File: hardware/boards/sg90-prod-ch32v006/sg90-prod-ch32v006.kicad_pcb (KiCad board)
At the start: 4 copper layers, 12.1 x 9.6 mm, 32 parts, among them J1 Servo Input, J2 Motor, J3 Debug, J4 Potentiometer, U1 H7133-1, U4 DRV8837, U5 CH32V006F8U6, U6 74LVC2G241GS,115

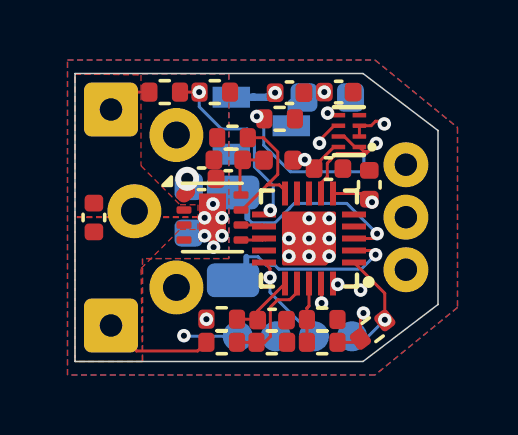
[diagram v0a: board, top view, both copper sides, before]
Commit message: rebuilt board
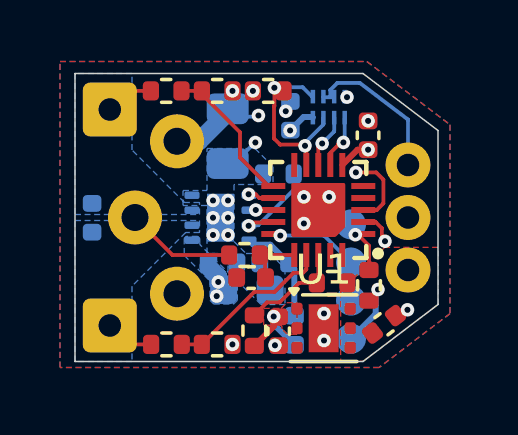
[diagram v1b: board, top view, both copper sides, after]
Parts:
- removed C3: 10µF, Capacitor_SMD:C_0402_1005Metric
- C1: value 10µF -> 1µF; footprint Capacitor_SMD:C_0603_1608Metric -> Capacitor_SMD:C_0402_1005Metric; moved to F.Cu
- C2: value 1µF -> 4.7µF
- C4, C7, C8, C9, FB1, R3, U4, U6: moved to B.Cu
- J4: moved to F.Cu
- NT1, NT2: footprint shared:NetTie-2_SMD_0.2mm -> shared:NetTie-2_SMD_0.127mm
- RS1: value 0.1Ω 1% -> 10mΩ 1%; footprint Resistor_SMD:R_1206_3216Metric -> Resistor_SMD:R_0805_2012Metric
- U1: value H7133-1 -> TLV76733DRVR; footprint shared:SOT-23-3_L2.9-W1.3-P1.90-LS2.4-BR -> Package_SON:WSON-6-1EP_2x2mm_P0.65mm_EP1x1.6mm; moved to F.Cu
- moved R7 8.58 mm to (103.0, 90.8)
- moved R8 8.58 mm to (104.7, 90.8)
- moved R6 8.41 mm to (104.7, 99.2)
- moved R5 8.41 mm to (103.0, 99.2)
- moved C2 8.22 mm to (106.8, 98.8), turned to -90 degrees
- moved C1 7.79 mm to (110.3, 98.6), turned to 37.235 degrees
- moved U1 7.06 mm to (108.3, 98.7), turned to 0 degrees
- moved FB1 5.69 mm to (107.3, 98.8), turned to 90 degrees
- moved NT2 4.87 mm to (105.9, 91.6), turned to 180 degrees
- moved C7 3.76 mm to (106.6, 96.5)
- moved RS1 3.34 mm to (105.1, 92.3), turned to -90 degrees
- moved C10 3.30 mm to (105.7, 97.4), turned to 0 degrees
- moved C9 2.88 mm to (104.9, 96.5)
- moved J3 2.61 mm to (109.2, 97.1), turned to 90 degrees
- moved R9 2.30 mm to (106.0, 98.8), turned to 90 degrees
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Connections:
- C2 pad 1: VSYS -> +3V3
- U1 pad 1: GND -> +3V3
- U1 pad 3: VSYS -> GND
- U5 pad 10: /EN -> unconnected-(U5-PC3/T1C3/T2C3_4-Pad10)
- U5 pad 11: /VSNA -> /VSNB
- U5 pad 12: /IN1 -> /IN2
- U5 pad 13: /IN2 -> /IN1
- U5 pad 14: unconnected-(U5-PC7-Pad14) -> /EN
- U5 pad 17: /VSNB -> /VSNA
- U5 pad 19: /RX -> unconnected-(U5-PD5/A5-Pad19)
- U5 pad 20: /TX -> unconnected-(U5-PD6/A6-Pad20)
- U5 pad 7: /TX_EN -> /TX
- U5 pad 8: unconnected-(U5-PC1/RX_3-Pad8) -> /RX
- U5 pad 9: unconnected-(U5-PC2/T2C2_2-Pad9) -> /TX_EN
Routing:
- net VSYS: track 15.1 -> 0.65 mm
- net /RX: track 7.85 -> 1.80 mm, vias 2 -> 1
- net /TX: track 6.83 -> 1.82 mm, vias 2 -> 1
- net /TX_EN: track 10.1 -> 6.10 mm
- net /ISNS-: track 5.46 -> 8.28 mm, vias 1 -> 2
- net /DATA: track 7.88 -> 5.21 mm, vias 1 -> 0
- net /nRST: track 3.68 -> 1.42 mm
- net GND: track 0.00 -> 2.21 mm, vias 9 -> 13
- net +3V3: track 8.57 -> 6.53 mm, vias 5 -> 4
- net /MOT_B: track 3.65 -> 1.79 mm
- net /3V3_DRV: track 1.92 -> 3.47 mm
- net /VNTC: track 1.99 -> 3.48 mm
- net /VSNB: track 3.56 -> 5.01 mm
- net /POT: track 5.00 -> 3.66 mm, vias 1 -> 0
- net /EN: track 4.43 -> 3.38 mm, vias 0 -> 1
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- added copper zone on F.Cu, net +3V3
- added copper zone on In2.Cu, net +3V3
- added copper zone on B.Cu, net /MOT_A
- added copper zone on B.Cu, net /MOT_B
- added copper zone on In1.Cu, net GND
- added copper zone on B.Cu, net VSYS
- added copper zone on F.Cu, net VSYS
- added copper zone on In2.Cu, net VSYS
- removed copper zone on In1.Cu, net +3V3
- removed copper zone on F.Cu, net /MOT_A
- removed copper zone on F.Cu, net /MOT_B
- removed copper zone on In2.Cu, net GND
- removed copper zone on F.Cu, net PGND
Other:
- board text removed: "+"
- board text removed: "-"
- board text removed: "A"
- board text removed: "B"
- board text removed: "D"
- board text removed: "R S G V"
- board text removed: "W"
